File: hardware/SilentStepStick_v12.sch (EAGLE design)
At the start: 30 parts, among them IC1 TMC2100_QFN36, X1 PASSER-07, X2 PASSER-07

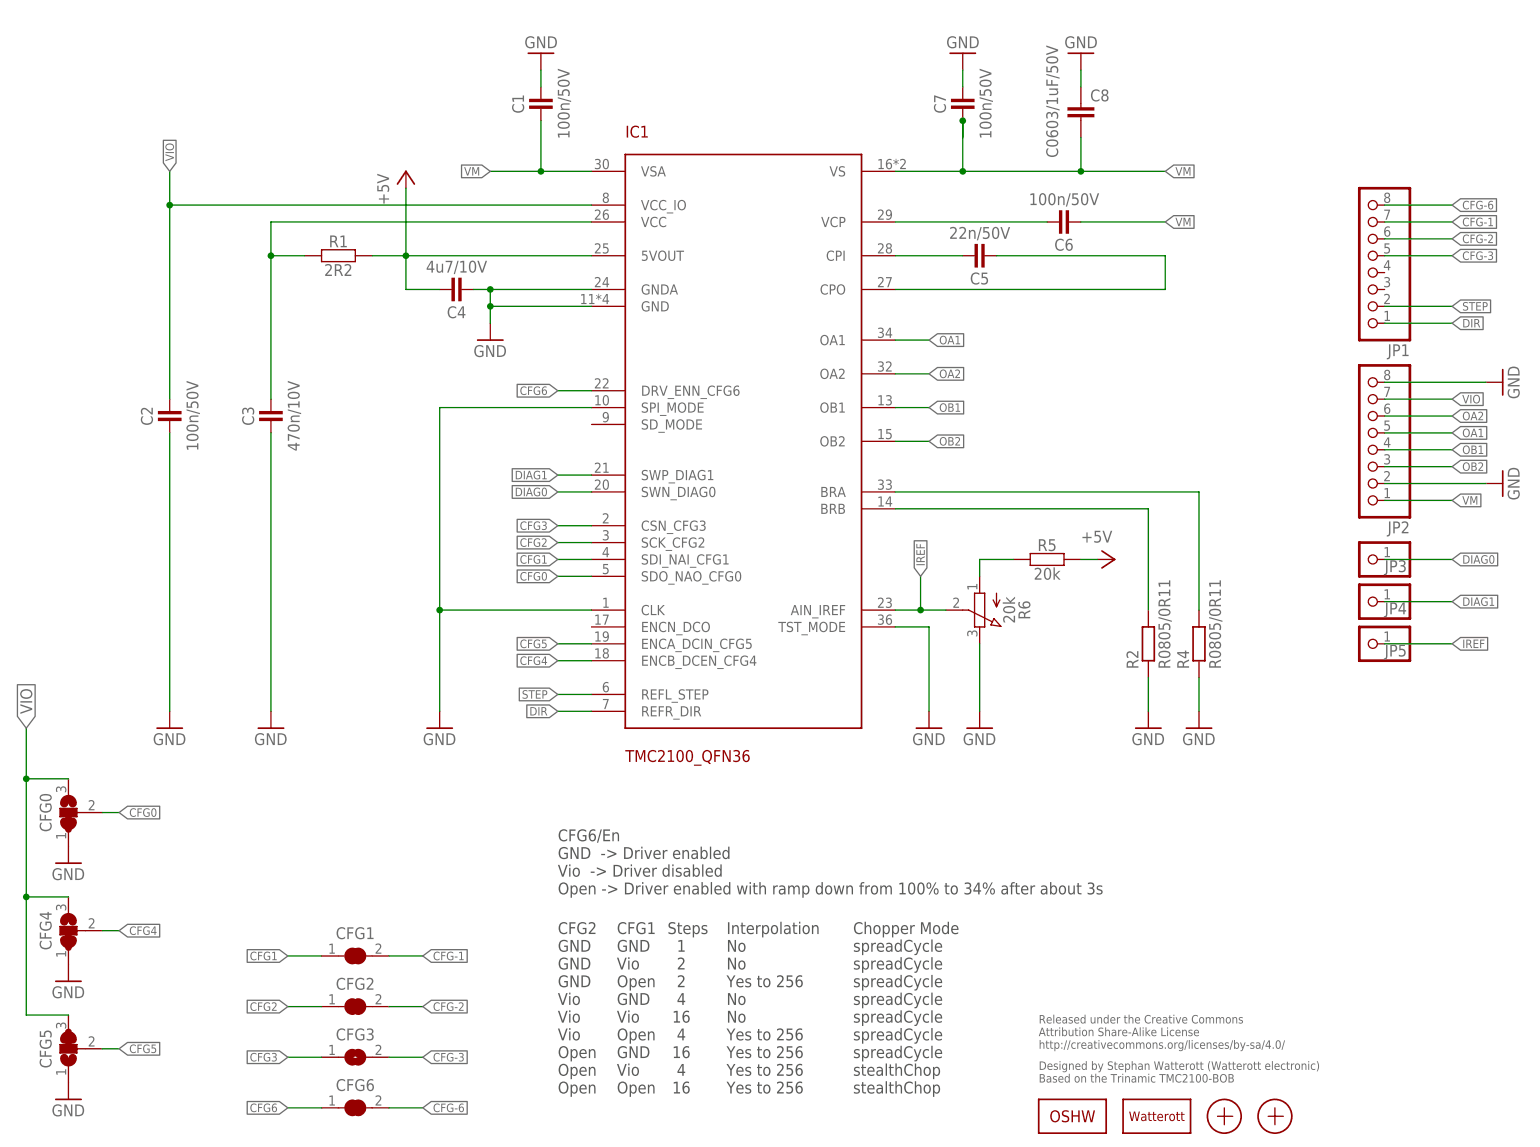
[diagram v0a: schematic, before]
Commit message: updated layout and schematics
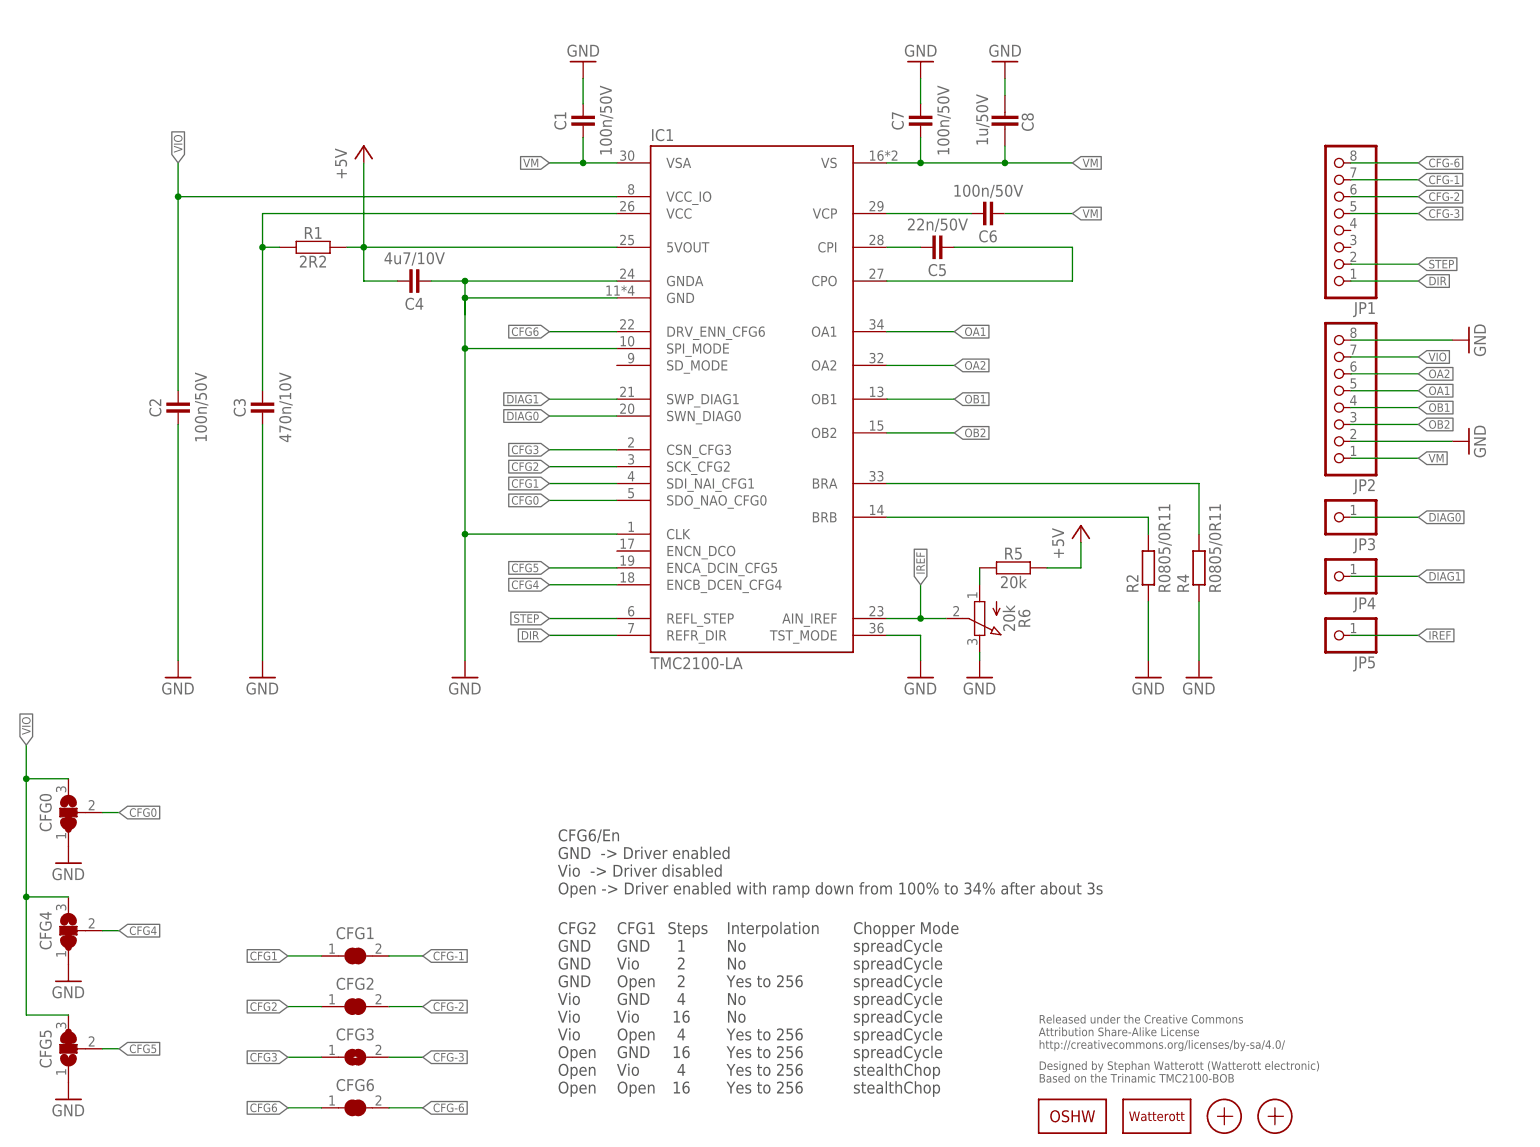
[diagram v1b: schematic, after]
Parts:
- C8: value C0603/1uF/50V -> 1u/50V
- IC1: value TMC2100_QFN36 -> TMC2100-LA; device TMC2100_QFN:TMC2100_QFN36 -> we-chip:TMC2100-LA
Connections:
- net N$7 renamed BRA
- net N$9 renamed BRB
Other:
- moved on the sheet: C1, C2, C3, C4, C5, C6, C7, C8, JP1, JP2, JP3, JP4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
